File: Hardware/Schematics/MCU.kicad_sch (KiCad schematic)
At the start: 31 parts, among them J5 Conn_ARM_SWD_TagConnect_TC2030, SW1 SW_Omron_B3FS, U2 CP2102N-Axx-xQFN28, U3 STM32WL55CCUx, Y1 SG-210STF 32MHz

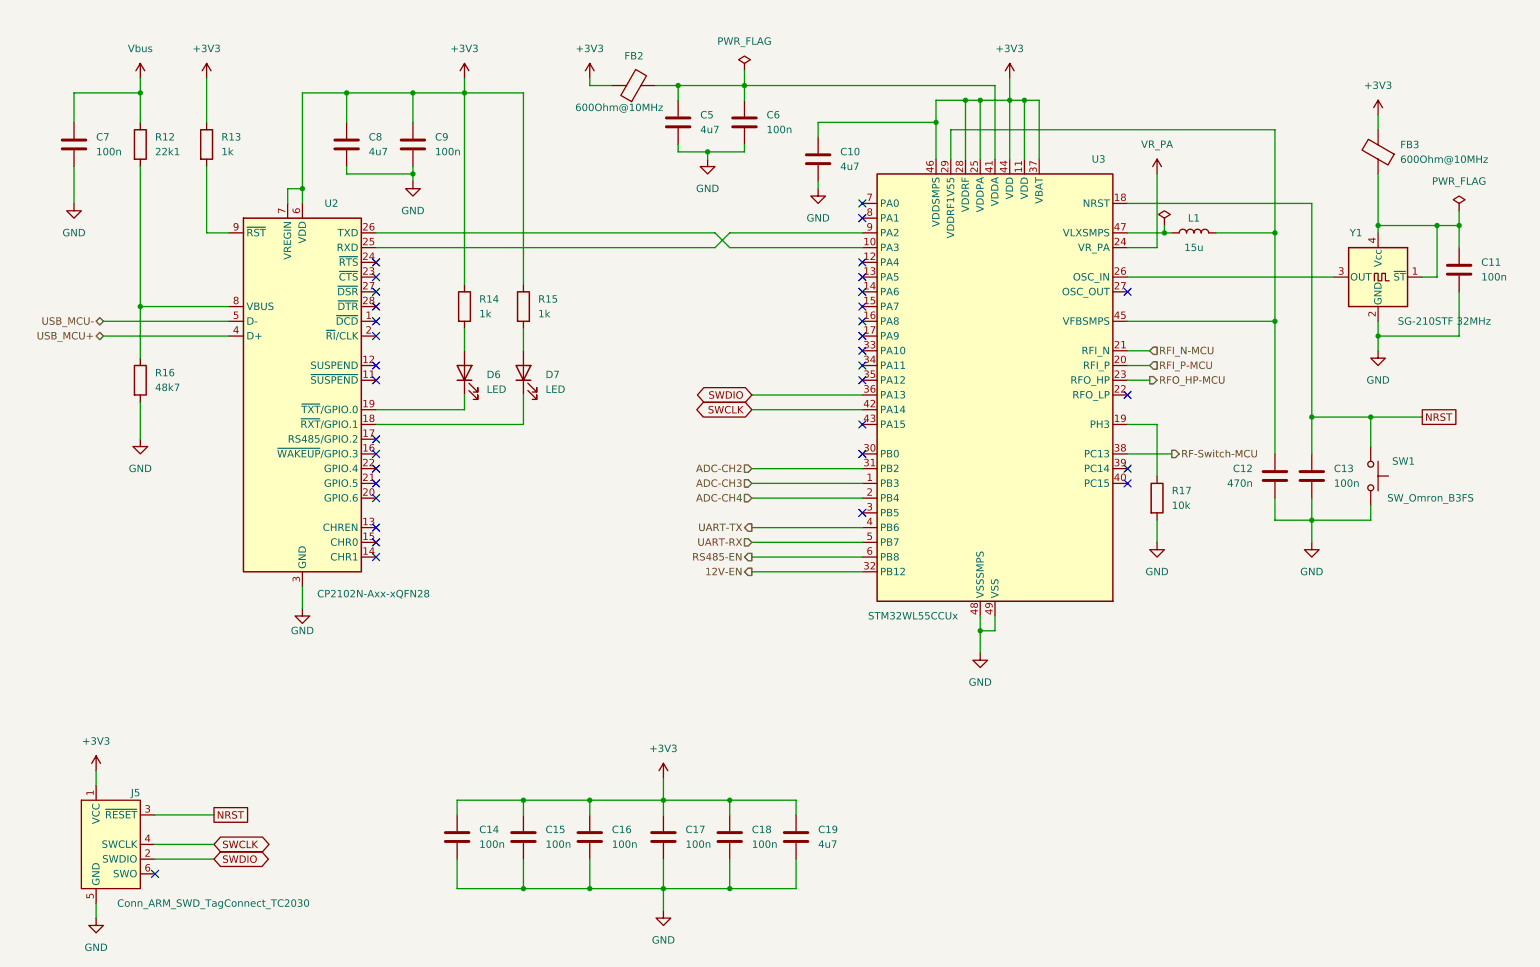
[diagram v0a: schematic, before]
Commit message: final hardware V1
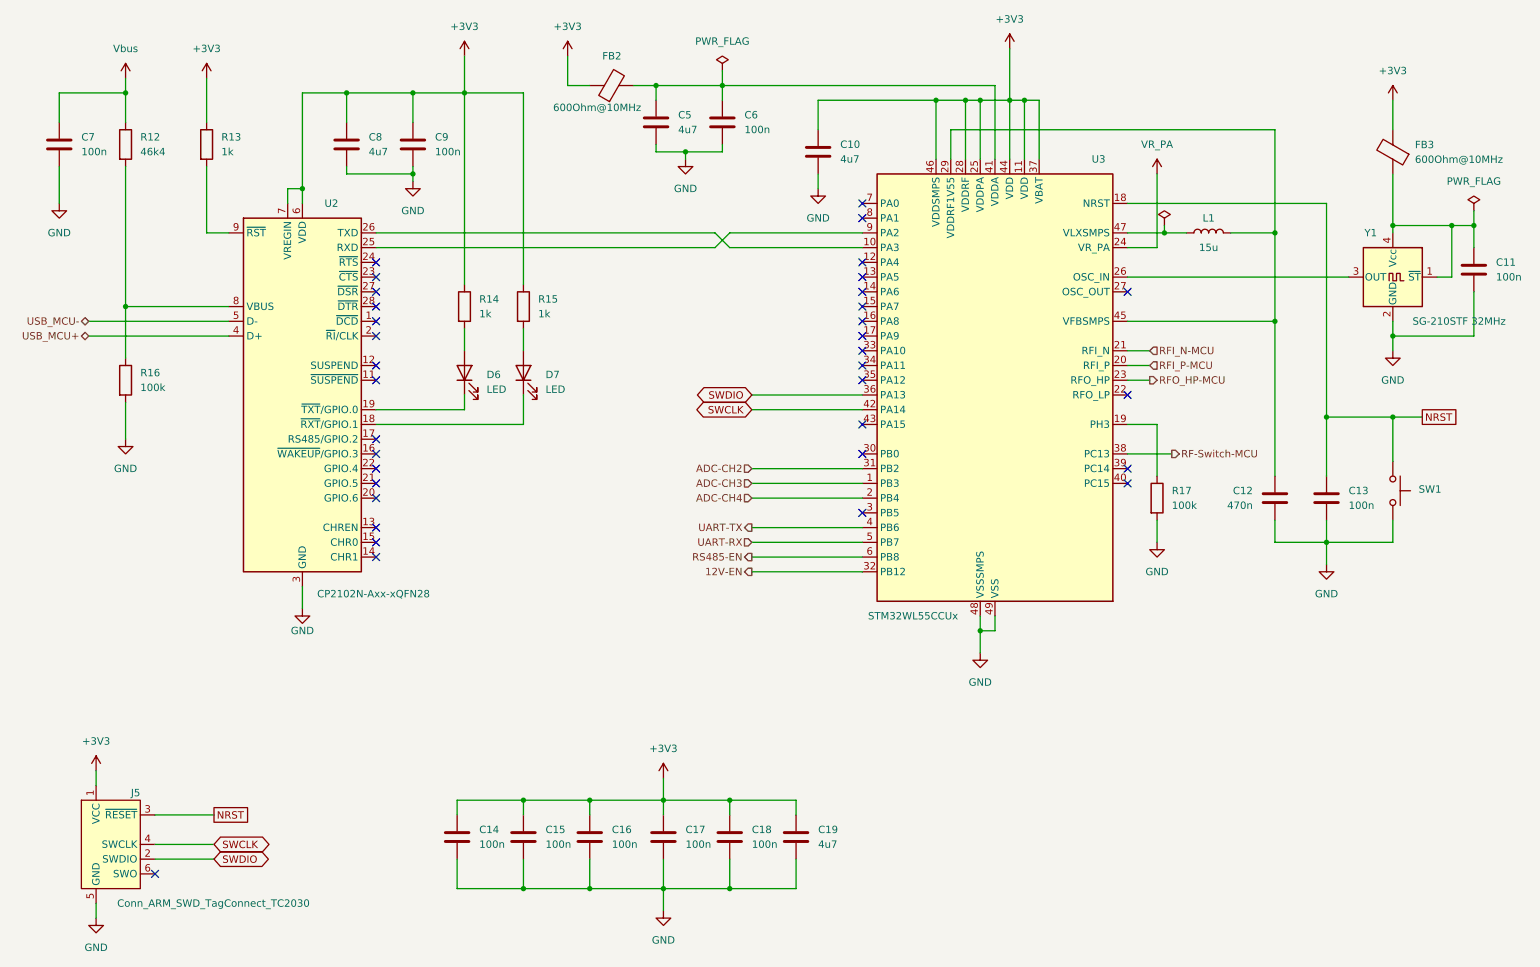
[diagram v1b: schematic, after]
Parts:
- R12: value 22k1 -> 46k4
- R16: value 48k7 -> 100k
- R17: value 10k -> 100k
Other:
- moved on the sheet: C10, C11, C12, C13, C5, C6, C7, FB2, FB3, L1, R12, R16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
